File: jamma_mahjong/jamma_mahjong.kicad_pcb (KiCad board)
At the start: 4 copper layers, 110.2 x 38.1 mm, 7 parts, among them J1 Jamma_Connector, J2 Mahjong_Connector, J3 Conn_02x07_Odd_Even, SW1 SW_SPDT

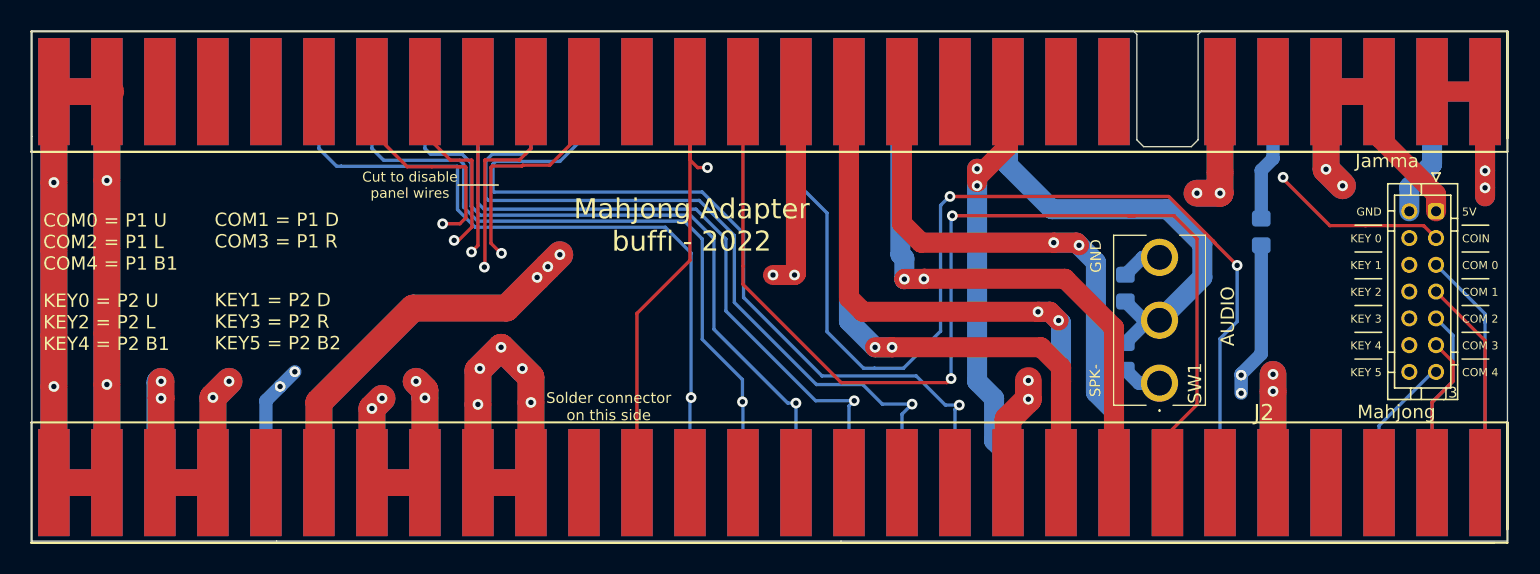
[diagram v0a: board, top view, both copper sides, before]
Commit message: v2
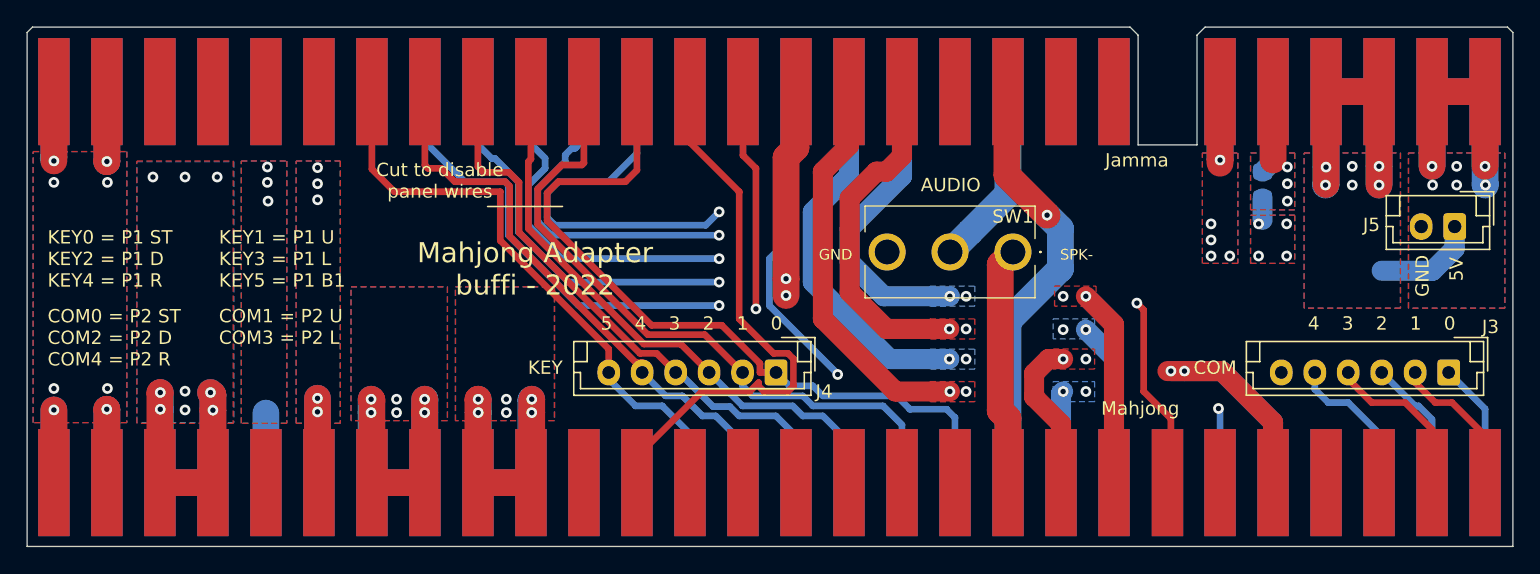
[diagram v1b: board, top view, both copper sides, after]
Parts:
- removed JMP2, JMP3: SolderJumper_2_Open, Resistor_SMD:R_0805_2012Metric_Pad1.20x1.40mm_HandSolder
- added J4: Conn_01x06, Connector_JST:JST_EH_B6B-EH-A_1x06_P2.50mm_Vertical, F.Cu at (176.8, 73.0)
- added J5: Conn_01x02, Connector_JST:JST_EH_B2B-EH-A_1x02_P2.50mm_Vertical, F.Cu at (227.4, 62.1)
- J3: value Conn_02x07_Odd_Even -> Conn_01x06; footprint Connector_JST:JST_PHD_B14B-PHDSS_2x07_P2.00mm_Vertical -> Connector_JST:JST_EH_B6B-EH-A_1x06_P2.50mm_Vertical
- moved SW1 14.7 mm to (194.4, 64.0), turned to -90 degrees
- moved J3 12.1 mm to (227.0, 73.0), turned to 180 degrees
- moved JMP1 3.50 mm to (213.1, 59.0)
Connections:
- J1 pad 11: Net-(J1-Pad11) -> unconnected-(J1-Pad11)
- J1 pad 17: Net-(J1-Pad17) -> KEY0-4
- J1 pad 18: COM0-3 -> KEY1-5
- J1 pad 19: COM1-2 -> KEY2-8
- J1 pad 20: COM2-6 -> KEY3-9
- J1 pad 21: COM3-10 -> KEY4-11
- J1 pad 22: COM4-7 -> KEY5-1
- J1 pad 23: Net-(J1-Pad23) -> unconnected-(J1-Pad23)
- J1 pad 24: Net-(J1-Pad24) -> unconnected-(J1-Pad24)
- J1 pad 25: Net-(J1-Pad25) -> unconnected-(J1-Pad25)
- J1 pad 26: Net-(J1-Pad26) -> unconnected-(J1-Pad26)
- J1 pad 5: Net-(J1-Pad5) -> -5V
- J1 pad 8: Net-(J1-Pad8) -> unconnected-(J1-Pad8)
- J1 pad 9: Net-(J1-Pad9) -> unconnected-(J1-Pad9)
- J1 pad J: Net-(J1-PadJ) -> unconnected-(J1-PadJ)
- J1 pad K: Net-(J1-PadK) -> unconnected-(J1-PadK)
- J1 pad M: Net-(J1-PadM) -> unconnected-(J1-PadM)
- J1 pad S: Net-(J1-PadS) -> unconnected-(J1-PadS)
- J1 pad T: Net-(J1-PadT) -> unconnected-(J1-PadT)
- J1 pad U: Net-(J1-PadU) -> COM0-3
- J1 pad V: KEY0-4 -> COM1-2
- J1 pad W: KEY1-5 -> COM2-6
- J1 pad X: KEY2-8 -> COM3-10
- J1 pad Y: KEY3-9 -> COM4-7
- J1 pad Z: KEY4-11 -> unconnected-(J1-PadZ)
- J1 pad a: KEY5-1 -> unconnected-(J1-Pada)
- J1 pad b: Net-(J1-Padb) -> unconnected-(J1-Padb)
- J1 pad c: Net-(J1-Padc) -> unconnected-(J1-Padc)
- J1 pad d: Net-(J1-Padd) -> unconnected-(J1-Padd)
- J2 pad 11: Net-(J2-Pad11) -> unconnected-(J2-Pad11)
- J2 pad 12: Net-(J2-Pad12) -> unconnected-(J2-Pad12)
- J2 pad 13: Net-(J2-Pad13) -> unconnected-(J2-Pad13)
- J2 pad 14: Net-(J2-Pad14) -> unconnected-(J2-Pad14)
- J2 pad 15: Net-(J2-Pad15) -> unconnected-(J2-Pad15)
- J2 pad 16: Net-(J2-Pad16) -> unconnected-(J2-Pad16)
- J2 pad 18: Net-(J2-Pad18) -> unconnected-(J2-Pad18)
- J2 pad 24: Net-(J2-Pad24) -> unconnected-(J2-Pad24)
- J2 pad 3: Net-(J2-Pad3) -> unconnected-(J2-Pad3)
- J2 pad 4: Net-(J2-Pad4) -> unconnected-(J2-Pad4)
- J2 pad 6: Net-(J2-Pad6) -> unconnected-(J2-Pad6)
- J2 pad D: Net-(J2-PadD) -> unconnected-(J2-PadD)
- J2 pad H: Net-(J2-PadH) -> unconnected-(J2-PadH)
- J2 pad U: Net-(J2-PadU) -> unconnected-(J2-PadU)
- J2 pad V: Net-(J2-PadV) -> unconnected-(J2-PadV)
- J3 pad 1: 5V -> COM0-3
- J3 pad 2: GND -> COM1-2
- J3 pad 3: COIN -> COM2-6
- J3 pad 4: KEY0-4 -> COM3-10
- J3 pad 5: COM0-3 -> COM4-7
- J3 pad 6: KEY1-5 -> unconnected-(J3-Pad6)
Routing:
- net GND: track 252.4 -> 150.3 mm, vias 15 -> 24
- net KEY5-1: track 115.6 -> 44.9 mm, vias 1 -> 0
- net KEY4-11: track 110.5 -> 43.4 mm, vias 1 -> 0
- net KEY3-9: track 105.3 -> 43.4 mm, vias 1 -> 0
- net KEY2-8: track 101.5 -> 43.9 mm, vias 1 -> 0
- net COIN: track 95.1 -> 42.3 mm, vias 2 -> 0
- net KEY1-5: track 103.0 -> 50.6 mm, vias 1 -> 0
- net KEY0-4: track 105.6 -> 57.2 mm, vias 1 -> 0
- net 12V: track 127.7 -> 98.1 mm, vias 5 -> 10
- net JAMMA_SPK-: track 35.9 -> 13.8 mm
- net SERVICE: track 81.1 -> 60.8 mm
- net TEST: track 83.9 -> 66.6 mm
- net COM4-7: track 113.7 -> 97.5 mm
- net COM2-6: track 109.4 -> 94.8 mm
- net COM1-2: track 112.2 -> 97.6 mm
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- added copper zone on B.Cu, net -5V
- added copper zone on F.Cu, net -5V
- added copper zone on B.Cu, net -5V_M
- added copper zone on F.Cu, net -5V_M
- added copper zone on In1.Cu, net -5V_M
- added copper zone on B.Cu, net 12V
- added copper zone on F.Cu, net 12V
- added copper zone on In1.Cu, net 12V
- added copper zone on B.Cu, net 5V
- added copper zone on F.Cu, net 5V
- added copper zone on B.Cu, net BLUE
- added copper zone on F.Cu, net BLUE
- added copper zone on In1.Cu, net BLUE
- added copper zone on B.Cu, net GND
- added copper zone on F.Cu, net GND
- added copper zone on B.Cu, net GREEN
- added copper zone on F.Cu, net GREEN
- added copper zone on In1.Cu, net GREEN
- added copper zone on B.Cu, net RED
- added copper zone on F.Cu, net RED
- added copper zone on In1.Cu, net RED
- added copper zone on B.Cu, net SYNC
- added copper zone on F.Cu, net SYNC
- added copper zone on In1.Cu, net SYNC
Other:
- board size 110.2 x 38.1 mm -> 111 x 38.8 mm
- net class Default removed
- board text added: "0"
- board text added: "1"
- board text added: "2"
- board text added: "3"
- board text added: "4"
- board text added: "5"
- board text added: "COM"
- board text added: "COM0 = P2 ST COM2 = P2 D COM4 = P2 R"
- board text added: "COM1 = P2 U COM3 = P2 L"
- board text added: "KEY"
- board text added: "KEY0 = P1 ST KEY2 = P1 D KEY4 = P1 R"
- board text added: "KEY1 = P1 U KEY3 = P1 L KEY5 = P1 B1"
- board text removed: "COIN"
- board text removed: "COM 0"
- board text removed: "COM 1"
- board text removed: "COM 2"
- board text removed: "COM 3"
- board text removed: "COM 4"
- board text removed: "COM0 = P1 U COM2 = P1 L COM4 = P1 B1"
- board text removed: "COM1 = P1 D COM3 = P1 R"
- board text removed: "GND SPK-"
- board text removed: "JONG SPK-"
- board text removed: "KEY 0"
- board text removed: "KEY 1"
- board text removed: "KEY 2"
- board text removed: "KEY 3"
- board text removed: "KEY 4"
- board text removed: "KEY 5"
- board text removed: "KEY0 = P2 U KEY2 = P2 L KEY4 = P2 B1"
- board text removed: "KEY1 = P2 D KEY3 = P2 R KEY5 = P2 B2"
